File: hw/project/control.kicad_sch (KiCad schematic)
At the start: 44 parts, among them SW1 BOOT0, SW2 RESET, U1 STSPIN32G4, X1 32MHZ 10PF

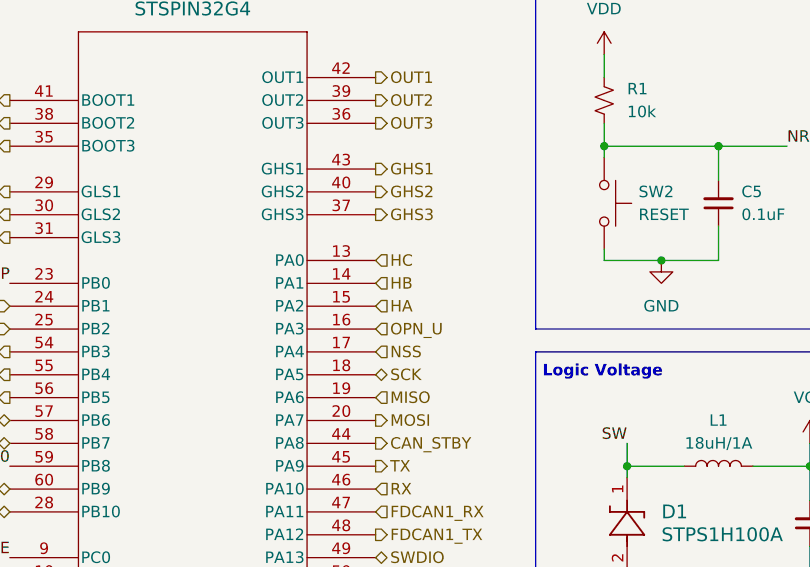
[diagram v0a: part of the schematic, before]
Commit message: Label everythangg
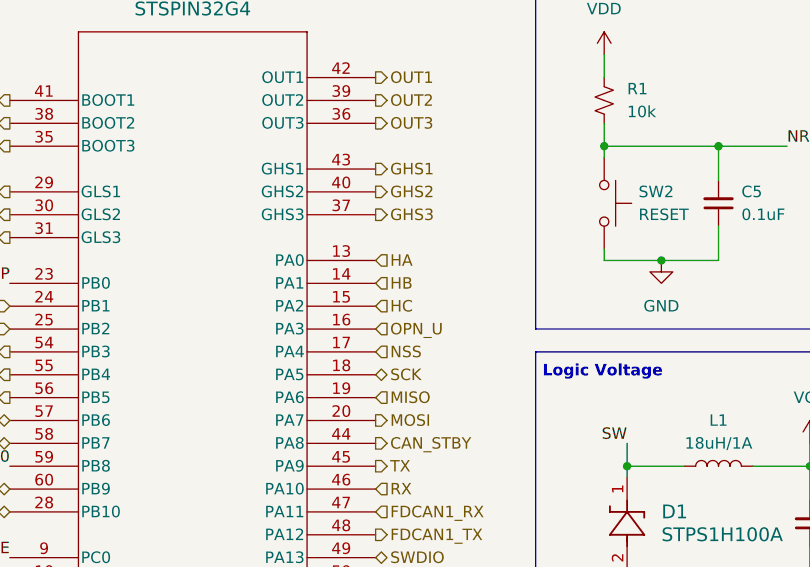
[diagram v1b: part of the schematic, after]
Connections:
- net HA: now also U1.13 (PA0); no longer U1.15 (PA2)
- net HC: now also U1.15 (PA2); no longer U1.13 (PA0)
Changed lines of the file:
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@@
 	(hierarchical_label "HC"
 		(shape input)
-		(at 73.66 45.72 0)
+		(at 73.66 50.8 0)
 		(effects
 			(font
@@
 	(hierarchical_label "HA"
 		(shape input)
-		(at 73.66 50.8 0)
+		(at 73.66 45.72 0)
 		(effects
 			(font
